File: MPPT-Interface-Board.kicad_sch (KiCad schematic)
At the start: 35 parts, among them J1 FIRST MPPT, J2 LAST MPPT, J3 CarCAN In, J4 CarCAN Out, J5 FUSEBOX, Q1 PMV35EPER, U1 RI3-1209S

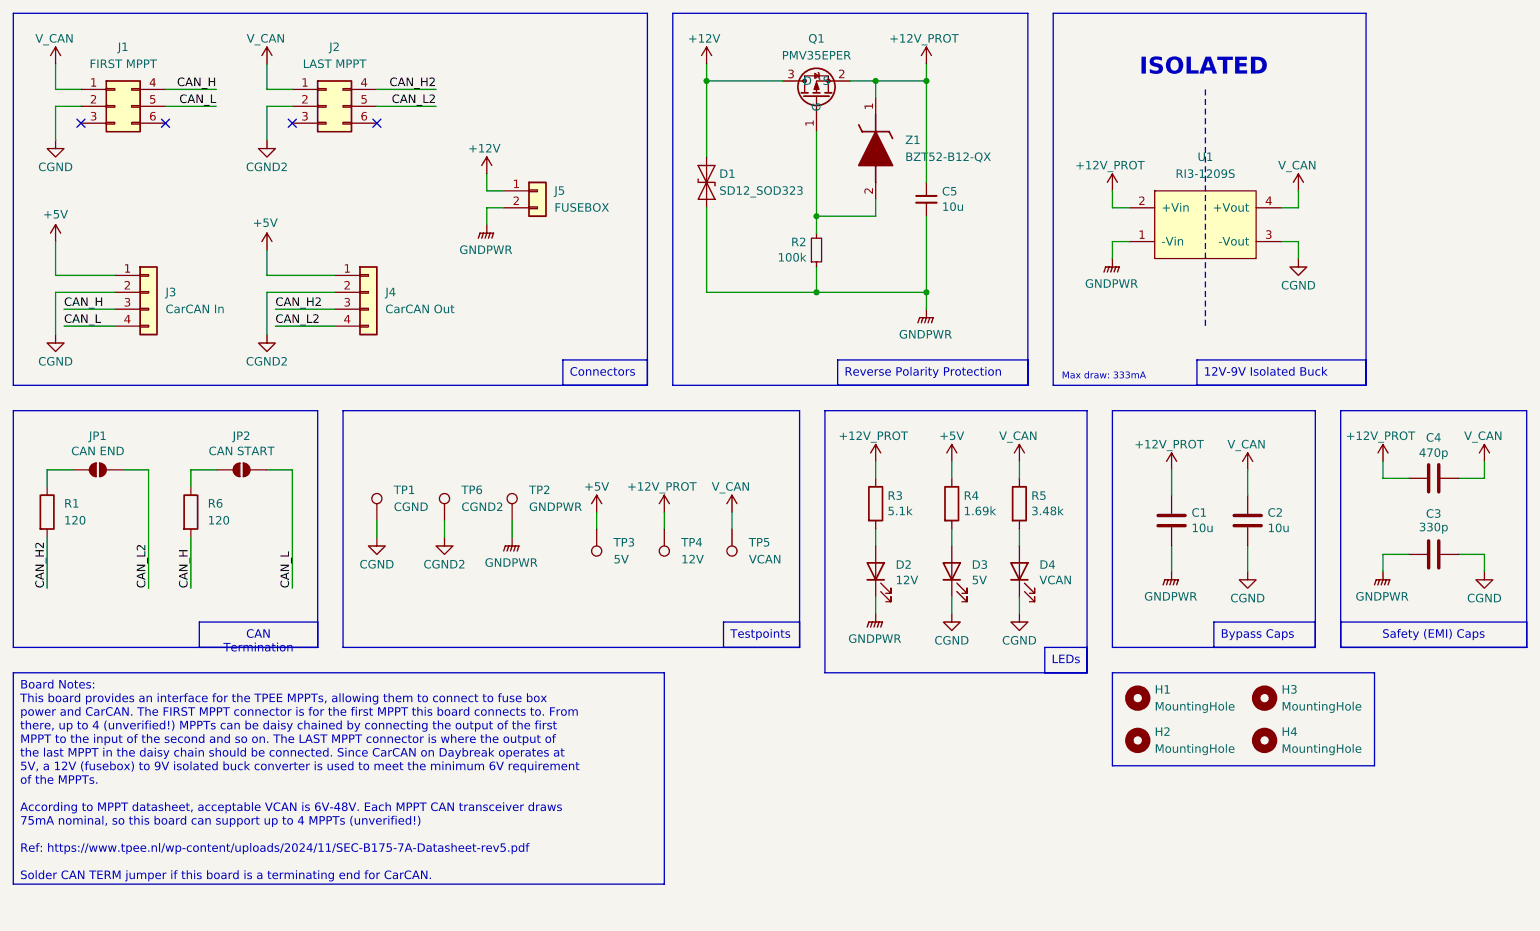
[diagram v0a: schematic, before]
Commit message: Changed up to interface data acq leader
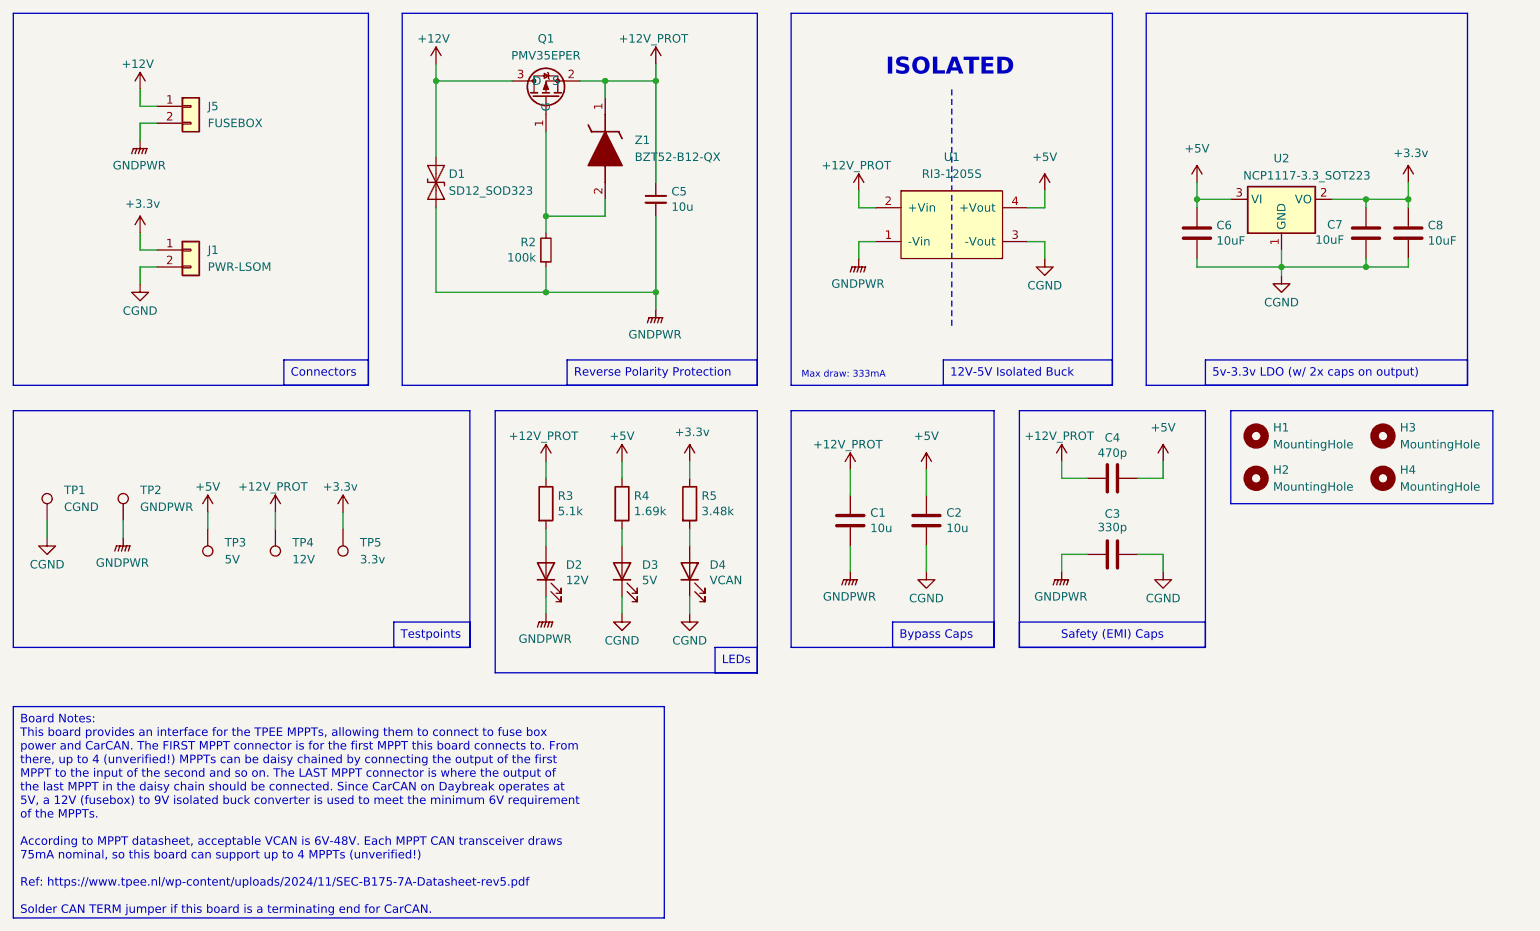
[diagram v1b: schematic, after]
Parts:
- removed J1: FIRST MPPT, Connector_Molex:Molex_Micro-Fit_3.0_43045-0612_2x03_P3.00mm_Vertical, symbol Connector_Generic:Conn_02x03_Top_Bottom
- removed J2: LAST MPPT, Connector_Molex:Molex_Micro-Fit_3.0_43045-0612_2x03_P3.00mm_Vertical, symbol Connector_Generic:Conn_02x03_Top_Bottom
- removed J3: CarCAN In, UTSVT-Connectors:Molex_MicroFit3.0_1x4xP3.00mm_PolarizingPeg_Vertical, symbol Connector_Generic:Conn_01x04
- removed J4: CarCAN Out, UTSVT-Connectors:Molex_MicroFit3.0_1x4xP3.00mm_PolarizingPeg_Vertical, symbol Connector_Generic:Conn_01x04
- removed JP1: CAN END, Jumper:SolderJumper-2_P1.3mm_Open_TrianglePad1.0x1.5mm, symbol Jumper:SolderJumper_2_Open
- removed JP2: CAN START, Jumper:SolderJumper-2_P1.3mm_Open_TrianglePad1.0x1.5mm, symbol Jumper:SolderJumper_2_Open
- removed R1, R6: 120, Resistor_SMD:R_0805_2012Metric, symbol Device:R
- removed TP6: CGND2, TestPoint:TestPoint_Pad_1.0x1.0mm, symbol Connector:TestPoint
- added C6, C7, C8: 10uF, Capacitor_SMD:C_0805_2012Metric, symbol Device:C
- added J1: PWR-LSOM, Connector_Molex:Molex_Micro-Fit_3.0_43650-0215_1x02_P3.00mm_Vertical, symbol Connector_Generic:Conn_01x02
- added U2: NCP1117-3.3_SOT223, Package_TO_SOT_SMD:SOT-223-3_TabPin2, symbol Regulator_Linear:LD1117S33TR_SOT223
- TP5: value VCAN -> 3.3v
- U1: value RI3-1209S -> RI3-1205S; Mouser Part Number (none) -> 919-RI3-1205S; Mouser Price/Stock (none) -> https://www.mouser.com/ProductDetail/RECOM-Power/RI3-1205S?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; P/N RI3-1209S -> RI3-1205S
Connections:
- net +5V: now also C2.1, C4.2, U1.4 (+Vout), C6.1, U2.3 (VI)
- net CGND: now also C6.2, C7.2, C8.2, J1.2 (Pin_2), U2.1 (GND)
- removed net V_CAN: C2.1, C4.2, R5.1, TP5.1, U1.4 (+Vout)
- new net +3.3v: C7.1, C8.1, J1.1 (Pin_1), R5.1, TP5.1, U2.2 (VO)
- no-connect marks 4 -> 0
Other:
- moved on the sheet: C1, C2, C3, C4, C5, D1, D2, D3, D4, H1, H2, H3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
